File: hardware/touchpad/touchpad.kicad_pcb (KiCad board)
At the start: 2 copper layers, 194.2 x 134.1 mm, 187 parts, among them J1 Conn_01x26_MountingPin, J10 Conn_02x03_Odd_Even, J100 Conn_02x03_Odd_Even, J101 Conn_02x03_Odd_Even, J102 Conn_02x03_Odd_Even, J103 Conn_02x03_Odd_Even, J104 Conn_02x03_Odd_Even, J105 Conn_02x03_Odd_Even, J106 Conn_02x03_Odd_Even, J107 Conn_02x03_Odd_Even, J108 Conn_02x03_Odd_Even, J109 Conn_02x03_Odd_Even, J11 Conn_02x03_Odd_Even, J110 Conn_02x03_Odd_Even, J111 Conn_02x03_Odd_Even, J112 Conn_02x03_Odd_Even, J113 Conn_02x03_Odd_Even, J114 Conn_02x03_Odd_Even, J115 Conn_02x03_Odd_Even, J116 Conn_02x03_Odd_Even, J117 Conn_02x03_Odd_Even, J118 Conn_02x03_Odd_Even, J119 Conn_02x03_Odd_Even, J12 Conn_02x03_Odd_Even, J120 Conn_02x03_Odd_Even, J121 Conn_02x03_Odd_Even, J122 Conn_02x03_Odd_Even, J123 Conn_02x03_Odd_Even, J124 Conn_02x03_Odd_Even, J125 Conn_02x03_Odd_Even, J126 Conn_02x03_Odd_Even, J127 Conn_02x03_Odd_Even, J128 Conn_02x03_Odd_Even, J129 Conn_02x03_Odd_Even, J13 Conn_02x03_Odd_Even, J130 Conn_02x03_Odd_Even, J131 Conn_02x03_Odd_Even, J132 Conn_02x03_Odd_Even, J133 Conn_02x03_Odd_Even, J134 Conn_02x03_Odd_Even, J135 Conn_02x03_Odd_Even, J136 Conn_02x03_Odd_Even, J137 Conn_02x03_Odd_Even, J138 Conn_02x03_Odd_Even, J139 Conn_02x03_Odd_Even, J14 Conn_02x03_Odd_Even, J140 Conn_02x03_Odd_Even, J141 Conn_02x03_Odd_Even, J142 Conn_02x03_Odd_Even, J143 Conn_02x03_Odd_Even, J144 Conn_02x03_Odd_Even, J145 Conn_02x03_Odd_Even, J146 Conn_02x03_Odd_Even, J147 Conn_02x03_Odd_Even, J148 Conn_02x03_Odd_Even, J149 Conn_02x03_Odd_Even, J15 Conn_02x03_Odd_Even, J150 Conn_02x03_Odd_Even, J151 Conn_02x03_Odd_Even, J152 Conn_02x03_Odd_Even, J153 Conn_02x03_Odd_Even, J154 Conn_02x03_Odd_Even, J155 Conn_02x03_Odd_Even, J156 Conn_02x03_Odd_Even, J157 Conn_02x03_Odd_Even, J158 Conn_02x03_Odd_Even, J159 Conn_02x03_Odd_Even, J16 Conn_02x03_Odd_Even, J160 Conn_02x03_Odd_Even, J161 Conn_02x03_Odd_Even, J162 Conn_02x03_Odd_Even, J163 Conn_02x03_Odd_Even, J164 Conn_02x03_Odd_Even, J165 Conn_02x03_Odd_Even, J166 Conn_02x03_Odd_Even, J167 Conn_02x03_Odd_Even, J168 Conn_02x03_Odd_Even, J169 Conn_02x03_Odd_Even, J17 Conn_02x03_Odd_Even, J170 Conn_02x03_Odd_Even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

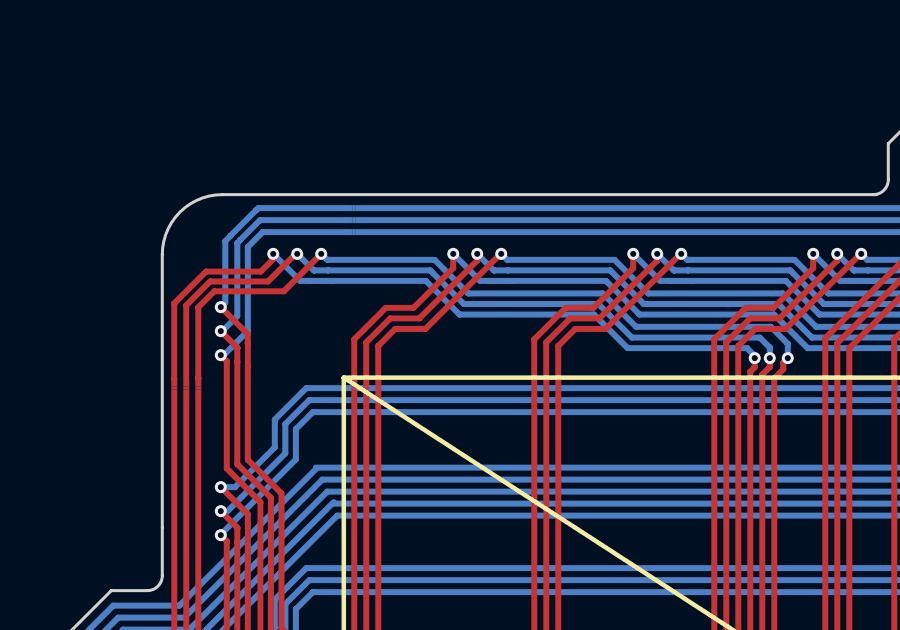
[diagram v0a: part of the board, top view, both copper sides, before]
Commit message: started schematics
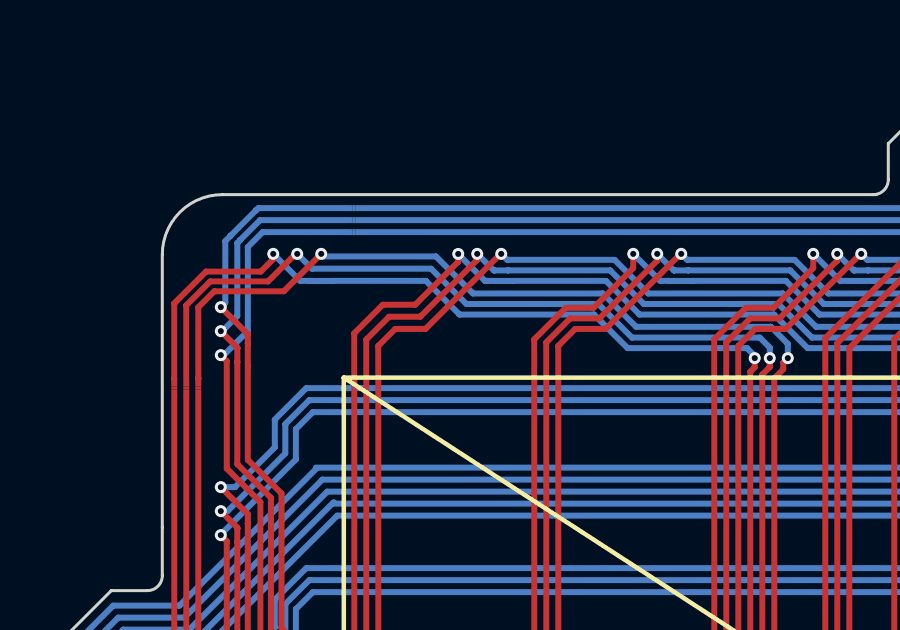
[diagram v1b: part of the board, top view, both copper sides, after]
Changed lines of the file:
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@@
 	)
 	(gr_rect
-		(start 60.05 92.1)
-		(end 64.55 78.6)
+		(start 60.05 78.6)
+		(end 64.55 92.1)
 		(stroke
 			(width 0.15)
@@
 	)
 	(gr_rect
-		(start 115.65 16.2)
-		(end 102.15 20.7)
+		(start 102.15 16.2)
+		(end 115.65 20.7)
 		(stroke
 			(width 0.15)
@@
 	)
 	(gr_rect
-		(start 60.05 60.7)
-		(end 64.55 47.2)
+		(start 60.05 47.2)
+		(end 64.55 60.7)
 		(stroke
 			(width 0.15)
@@
 	)
 	(segment
-		(start 97.601392 32.9)
-		(end 97.601392 33.145997)
+		(start 78.097389 33.569293)
+		(end 78.097389 32.282611)
 		(width 0.2)
 		(layer "F.Cu")
@@
 	)
 	(segment
-		(start 79.871389 31.576)
-		(end 81.797389 29.65)
+		(start 97.601392 32.9)
+		(end 97.601392 33.145997)
 		(width 0.2)
 		(layer "F.Cu")
@@
 	)
 	(segment
-		(start 78.097389 32.375)
-		(end 78.896389 31.576)
+		(start 97.601392 33.145997)
+		(end 97.298096 33.449293)
 		(width 0.2)
 		(layer "F.Cu")
@@
 	)
 	(segment
-		(start 78.097389 33.569293)
-		(end 78.097389 32.375)
+		(start 78.86 31.52)
+		(end 79.9 31.52)
 		(width 0.2)
 		(layer "F.Cu")
@@
 	)
 	(segment
-		(start 97.601392 33.145997)
-		(end 97.298096 33.449293)
+		(start 81.797389 29.622611)
+		(end 81.797389 29.425)
 		(width 0.2)
 		(layer "F.Cu")
@@
 	)
 	(segment
-		(start 81.797389 29.65)
-		(end 81.797389 29.425)
+		(start 79.9 31.52)
+		(end 81.797389 29.622611)
 		(width 0.2)
 		(layer "F.Cu")
@@
 	)
 	(segment
-		(start 78.896389 31.576)
-		(end 79.871389 31.576)
+		(start 78.097389 32.282611)
+		(end 78.86 31.52)
 		(width 0.2)
 		(layer "F.Cu")
@@
 	)
 	(segment
-		(start 96.897389 33.575)
-		(end 96.897389 33.599293)
+		(start 79.73 31.12)
+		(end 78.65 31.12)
 		(width 0.2)
 		(layer "F.Cu")
@@
 	)
 	(segment
-		(start 79.672389 31.225)
-		(end 80.997389 29.9)
+		(start 81.164165 29.427109)
+		(end 81.164165 29.685835)
 		(width 0.2)
 		(layer "F.Cu")
@@
 	)
 	(segment
-		(start 97.047389 33.203612)
-		(end 97.047389 32.824293)
+		(start 96.897389 33.575)
+		(end 96.897389 33.599293)
 		(width 0.2)
 		(layer "F.Cu")
@@
 	)
 	(segment
-		(start 77.697389 33.569293)
-		(end 77.697389 32.275)
+		(start 77.697389 32.072611)
+		(end 77.697389 33.597389)
 		(width 0.2)
 		(layer "F.Cu")
@@
 	)
 	(segment
-		(start 77.697389 32.275)
-		(end 78.747389 31.225)
+		(start 97.047389 33.203612)
+		(end 97.047389 32.824293)
 		(width 0.2)
 		(layer "F.Cu")
@@
 	)
 	(segment
-		(start 77.698096 33.57)
-		(end 77.697389 33.569293)
+		(start 96.898096 33.352905)
+		(end 97.047389 33.203612)
 		(width 0.2)
 		(layer "F.Cu")
@@
 	)
 	(segment
-		(start 96.898096 33.352905)
-		(end 97.047389 33.203612)
+		(start 78.65 31.12)
+		(end 77.697389 32.072611)
 		(width 0.2)
 		(layer "F.Cu")
@@
 	)
 	(segment
-		(start 80.997389 29.9)
-		(end 80.997389 29.425)
+		(start 81.164165 29.685835)
+		(end 79.73 31.12)
 		(width 0.2)
 		(layer "F.Cu")
@@
 	)
 	(segment
-		(start 78.747389 31.225)
-		(end 79.672389 31.225)
+		(start 77.697389 33.597389)
+		(end 77.7 33.6)
 		(width 0.2)
 		(layer "F.Cu")
@@
 	)
 	(via
-		(at 80.997389 29.425)
+		(at 81.164165 29.427109)
 		(size 0.4)
 		(drill 0.2)
@@
 	)
 	(segment
-		(start 82.97201 30.326)
-		(end 86.085613 30.326)
+		(start 82.201 30.325)
+		(end 82.202001 30.326)
 		(width 0.2)
 		(layer "B.Cu")
@@
 	)
 	(segment
-		(start 92.810751 32.566)
-		(end 96.789096 32.566)
+		(start 82.223769 30.327)
+		(end 82.971009 30.327)
 		(width 0.2)
 		(layer "B.Cu")
@@
 	)
 	(segment
-		(start 81.897389 30.325)
-		(end 82.201 30.325)
+		(start 81.164165 29.434165)
+		(end 82.055 30.325)
 		(width 0.2)
 		(layer "B.Cu")
@@
 	)
 	(segment
-		(start 82.222768 30.326)
-		(end 82.223769 30.327)
+		(start 91.691751 31.447)
+		(end 92.810751 32.566)
 		(width 0.2)
 		(layer "B.Cu")
@@
 	)
 	(segment
-		(start 82.201 30.325)
-		(end 82.202001 30.326)
+		(start 86.085613 30.326)
+		(end 87.206613 31.447)
 		(width 0.2)
 		(layer "B.Cu")
@@
 	)
 	(segment
-		(start 82.223769 30.327)
-		(end 82.971009 30.327)
+		(start 82.971009 30.327)
+		(end 82.97201 30.326)
 		(width 0.2)
 		(layer "B.Cu")
@@
 	)
 	(segment
-		(start 82.971009 30.327)
-		(end 82.97201 30.326)
+		(start 82.97201 30.326)
+		(end 86.085613 30.326)
 		(width 0.2)
 		(layer "B.Cu")
@@
 	)
 	(segment
-		(start 91.691751 31.447)
-		(end 92.810751 32.566)
+		(start 82.222768 30.326)
+		(end 82.223769 30.327)
 		(width 0.2)
 		(layer "B.Cu")
@@
 	)
 	(segment
-		(start 80.997389 29.425)
-		(end 81.897389 30.325)
+		(start 81.164165 29.427109)
+		(end 81.164165 29.434165)
 		(width 0.2)
 		(layer "B.Cu")
@@
 	)
 	(segment
-		(start 86.085613 30.326)
-		(end 87.206613 31.447)
+		(start 82.055 30.325)
+		(end 82.201 30.325)
+		(width 0.2)
+		(layer "B.Cu")
+		(net 345)
+	)
+	(segment
+		(start 92.810751 32.566)
+		(end 96.789096 32.566)
 		(width 0.2)
 		(layer "B.Cu")
@@
 	)
 	(segment
-		(start 80.231001 29.975)
-		(end 76.826621 29.975)
-		(width 0.2)
-		(layer "B.Cu")
-		(net 353)
-	)
-	(segment
-		(start 76.368157 29.975)
-		(end 76.347389 29.975)
-		(width 0.2)
-		(layer "B.Cu")
-		(net 353)
-	)
-	(segment
-		(start 91.217328 32.215)
-		(end 86.95614 32.215)
-		(width 0.2)
-		(layer "B.Cu")
-		(net 353)
-	)
-	(segment
 		(start 91.55 32.9)
 		(end 91.55 32.547672)
@@
 	)
 	(segment
-		(start 76.825621 29.976)
-		(end 76.369157 29.976)
-		(width 0.2)
-		(layer "B.Cu")
-		(net 353)
-	)
-	(segment
 		(start 86.95614 32.215)
 		(end 85.83714 31.096)
@@
 	)
 	(segment
-		(start 76.826621 29.975)
-		(end 76.825621 29.976)
+		(start 76.292389 29.92)
+		(end 75.797389 29.425)
 		(width 0.2)
 		(layer "B.Cu")
@@
 	)
 	(segment
-		(start 76.369157 29.976)
-		(end 76.368157 29.975)
+		(start 91.217328 32.215)
+		(end 86.95614 32.215)
 		(width 0.2)
 		(layer "B.Cu")
@@
 	)
 	(segment
-		(start 76.347389 29.975)
-		(end 75.797389 29.425)
+		(start 85.83714 31.096)
+		(end 81.436 31.096)
 		(width 0.2)
 		(layer "B.Cu")
@@
 	)
 	(segment
-		(start 81.352001 31.096)
-		(end 80.231001 29.975)
+		(start 81.436 31.096)
+		(end 80.26 29.92)
 		(width 0.2)
 		(layer "B.Cu")
@@
 	)
 	(segment
-		(start 85.83714 31.096)
-		(end 81.352001 31.096)
+		(start 80.26 29.92)
+		(end 76.292389 29.92)
 		(width 0.2)
 		(layer "B.Cu")
@@
 	)
 	(segment
-		(start 76.625959 29.425)
-		(end 76.597389 29.425)
+		(start 92.15 32.423379)
+		(end 91.582328 31.855707)
 		(width 0.2)
 		(layer "B.Cu")
@@
 	)
 	(segment
-		(start 85.982529 30.745)
-		(end 81.497389 30.745)
+		(start 80.42028 29.51)
+		(end 76.682389 29.51)
 		(width 0.2)
 		(layer "B.Cu")
@@
 	)
 	(segment
-		(start 92.15 32.423379)
-		(end 91.582328 31.855707)
+		(start 76.682389 29.51)
+		(end 76.597389 29.425)
 		(width 0.2)
 		(layer "B.Cu")
@@
 	)
 	(segment
-		(start 76.796389 29.624)
+		(start 76.625959 29.425)
 		(end 76.597389 29.425)
 		(width 0.2)
@@
 	)
 	(segment
-		(start 91.582328 31.855707)
-		(end 87.093236 31.855707)
+		(start 92.15 32.9)
+		(end 92.15 32.423379)
 		(width 0.2)
 		(layer "B.Cu")
@@
 	)
 	(segment
-		(start 80.376389 29.624)
-		(end 76.796389 29.624)
+		(start 81.65528 30.745)
+		(end 80.42028 29.51)
 		(width 0.2)
 		(layer "B.Cu")
@@
 	)
 	(segment
-		(start 81.497389 30.745)
-		(end 80.376389 29.624)
+		(start 87.093236 31.855707)
+		(end 85.982529 30.745)
 		(width 0.2)
 		(layer "B.Cu")
@@
 	)
 	(segment
-		(start 92.15 32.9)
-		(end 92.15 32.423379)
+		(start 91.582328 31.855707)
+		(end 87.093236 31.855707)
 		(width 0.2)
 		(layer "B.Cu")
@@
 	)
 	(segment
-		(start 87.093236 31.855707)
-		(end 85.982529 30.745)
+		(start 85.982529 30.745)
+		(end 81.65528 30.745)
 		(width 0.2)
 		(layer "B.Cu")

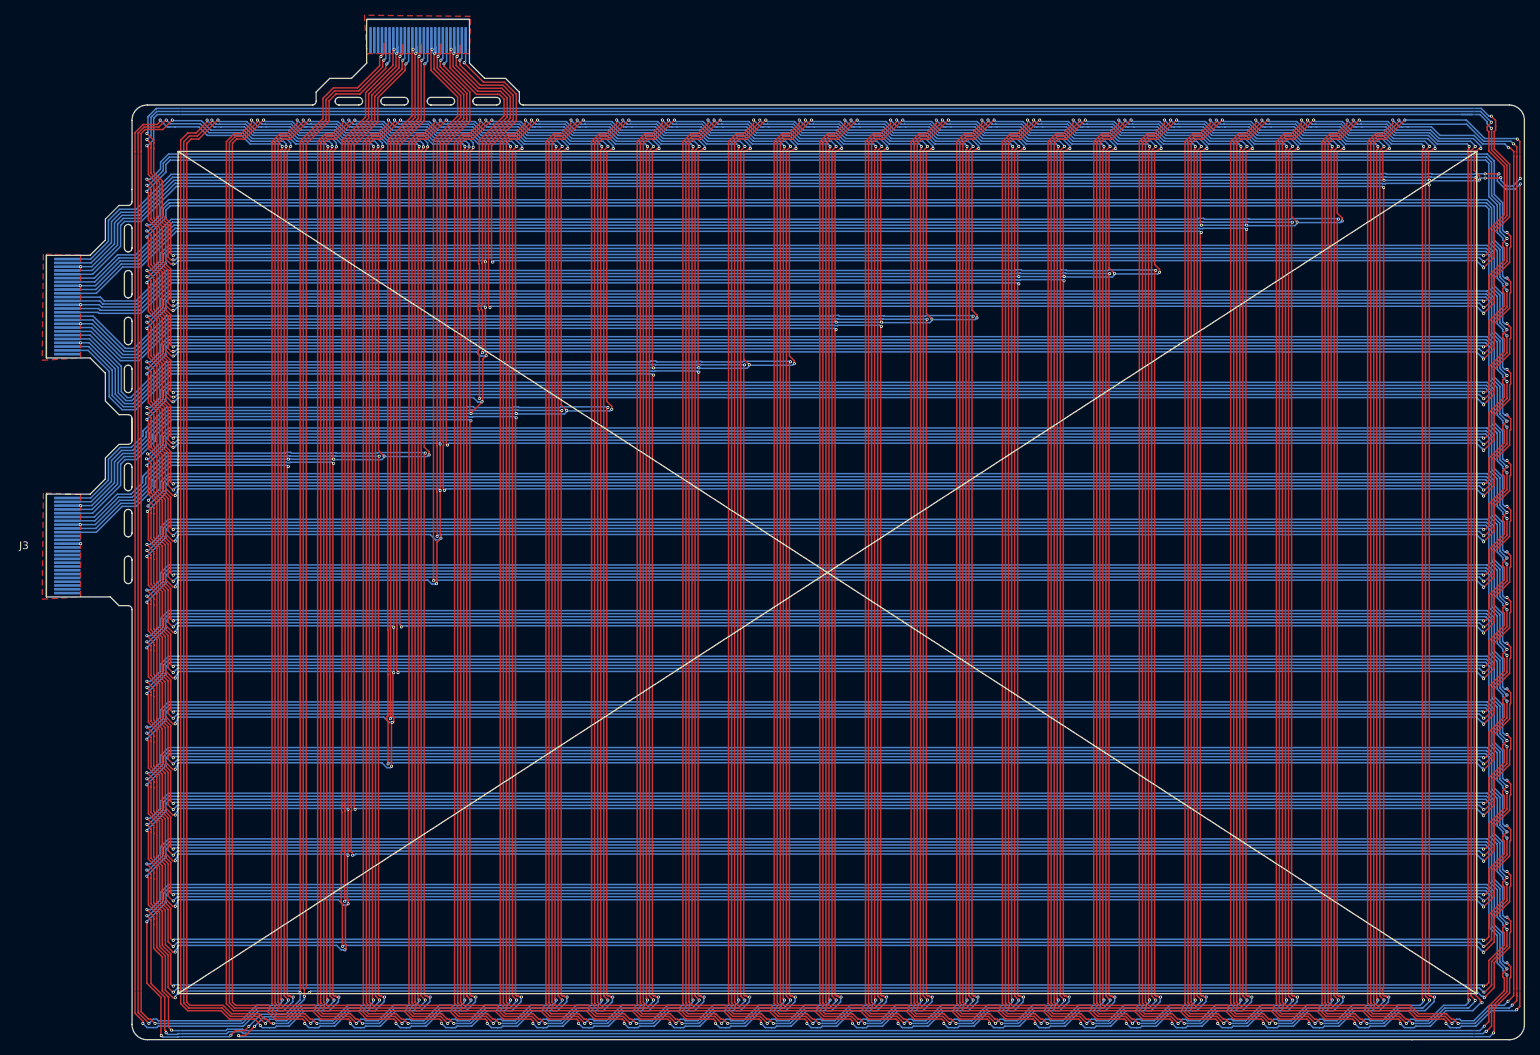
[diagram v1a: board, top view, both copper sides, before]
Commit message: fixed stuff
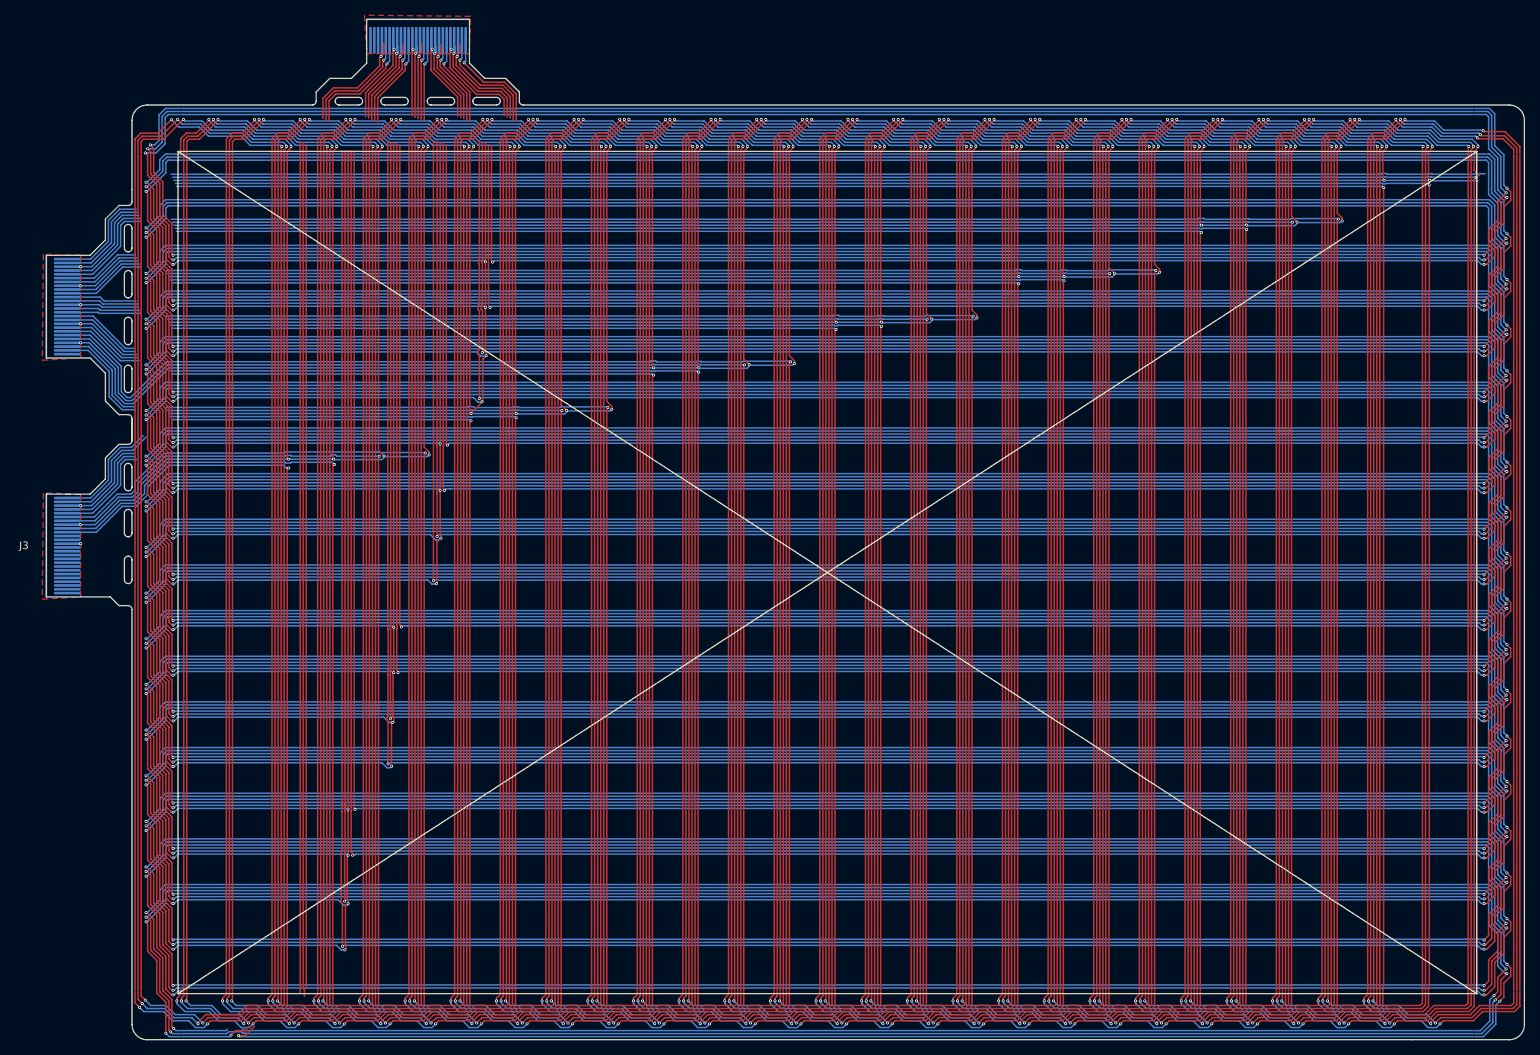
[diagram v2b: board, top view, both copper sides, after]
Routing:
- net /Y16: track 284.8 -> 127.6 mm, vias 2 -> 1
- net Net-(J105-Pin_6): track 109.4 -> 0.00 mm
- net GND: track 2509.0 -> 2419.2 mm, vias 62 -> 56
- net /Y17: track 306.4 -> 293.7 mm, vias 4 -> 2
- net /X0: track 306.2 -> 296.6 mm, vias 3 -> 0
- net /X23: track 135.9 -> 128.8 mm
- net /X22: track 142.2 -> 135.1 mm
- net /X7: track 253.0 -> 246.3 mm
- net /X18: track 172.4 -> 165.7 mm
- net /X19: track 166.0 -> 159.3 mm
- net /X6: track 259.3 -> 252.6 mm
- net /X5: track 266.1 -> 259.5 mm
- net /X4: track 272.7 -> 266.1 mm
- net /X2: track 292.2 -> 285.6 mm
- net /X3: track 285.8 -> 279.3 mm
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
